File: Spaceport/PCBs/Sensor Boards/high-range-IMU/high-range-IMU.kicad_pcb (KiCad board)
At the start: 2 copper layers, 19.5 x 21.5 mm, 4 parts, among them J1 Conn_01x06, U1 ADXL375BCCZ-RL7

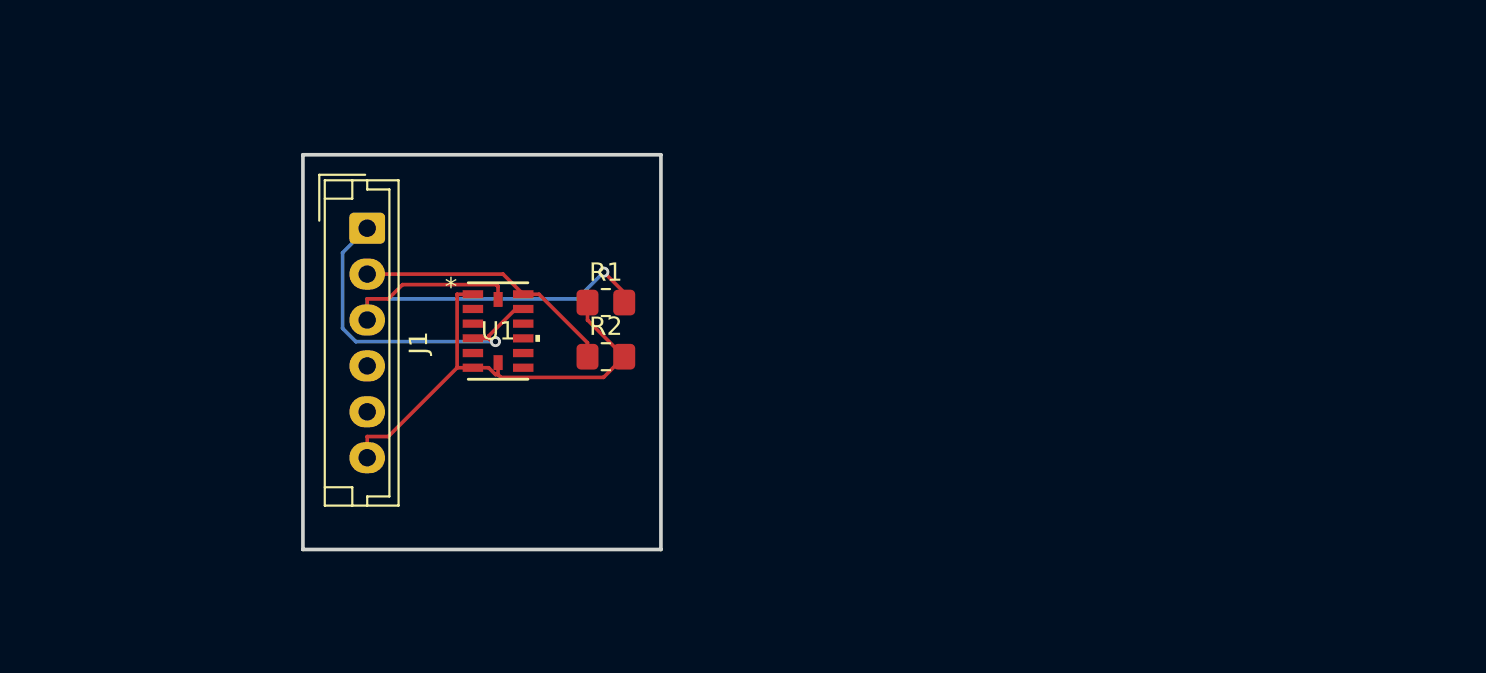
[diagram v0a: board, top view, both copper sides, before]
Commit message: Finished
Don't know if i did the ground plane correct. Don't know if I did the decoupling capacitor circuit correct.
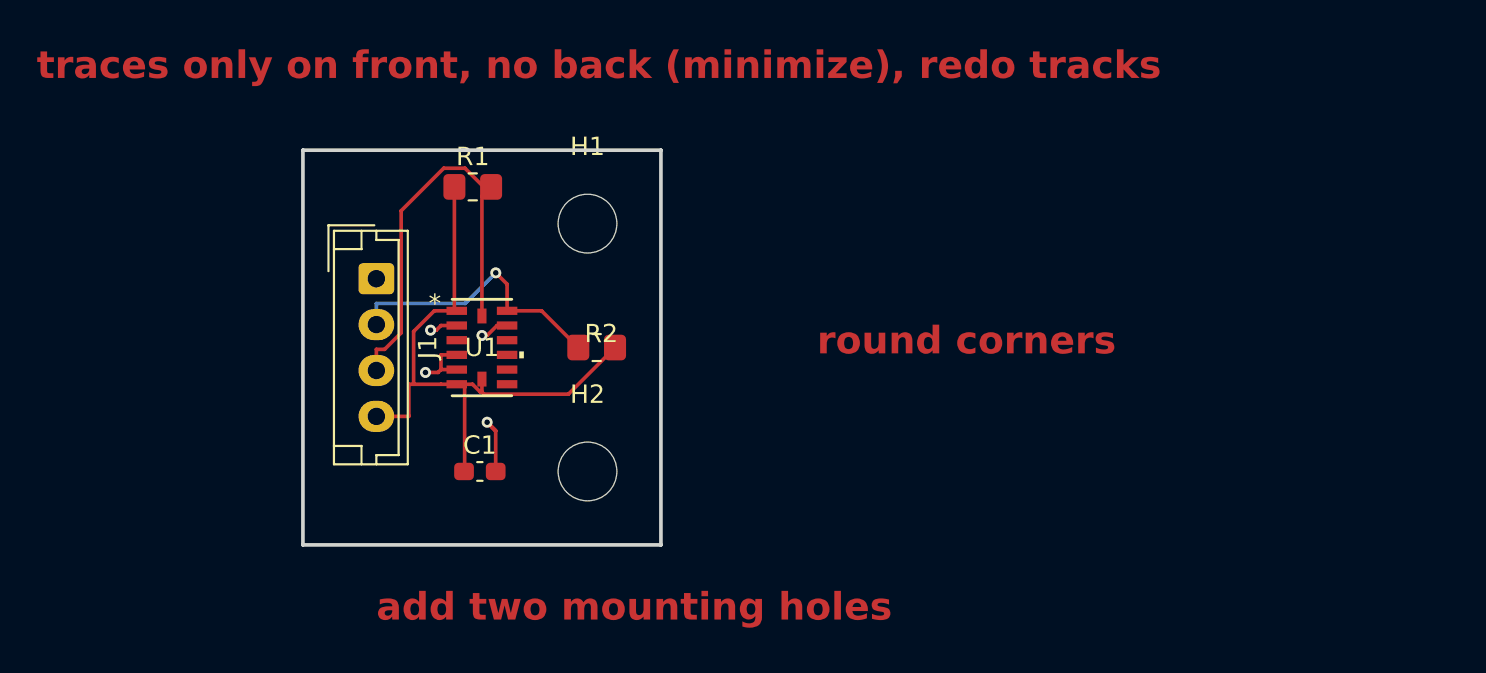
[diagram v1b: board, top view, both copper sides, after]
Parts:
- added C1: C, Capacitor_SMD:C_0603_1608Metric_Pad1.08x0.95mm_HandSolder, F.Cu at (144.6, 95.2)
- added H1: MountingHole, MountingHole:MountingHole_3.2mm_M3, F.Cu at (150.5, 81.8)
- added H2: MountingHole, MountingHole:MountingHole_3.2mm_M3, F.Cu at (150.5, 95.2)
- J1: value Conn_01x06 -> Conn_01x04; footprint Connector_JST:JST_EH_B6B-EH-A_1x06_P2.50mm_Vertical -> Connector_JST:JST_EH_B4B-EH-A_1x04_P2.50mm_Vertical
- moved R1 9.60 mm to (144.2, 79.8)
- moved J1 2.80 mm to (139.0, 84.8)
- moved U1 1.26 mm to (144.8, 88.5)
- moved R2 0.71 mm to (151.0, 88.5)
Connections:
- J1 pad 4: unconnected-(J1-Pin_4-Pad4) -> +3.3V
- U1 pad 2: unconnected-(U1-GND-Pad2) -> GND
- U1 pad 5: unconnected-(U1-GND-Pad5) -> GND
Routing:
- net GND: track 19.4 -> 11.4 mm, vias 1 -> 4
- net +3.3V: track 26.7 -> 33.9 mm
- net Net-(J1-Pin_3): track 26.1 -> 22.9 mm, vias 1 -> 0
- net Net-(J1-Pin_2): track 14.3 -> 15.4 mm, vias 0 -> 1
- added copper zone on B.Cu, net GND
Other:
- board text added: "add two mounting holes"
- board text added: "round corners"
- board text added: "traces only on front, no back (minimize), redo tracks"

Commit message: update PCB layout
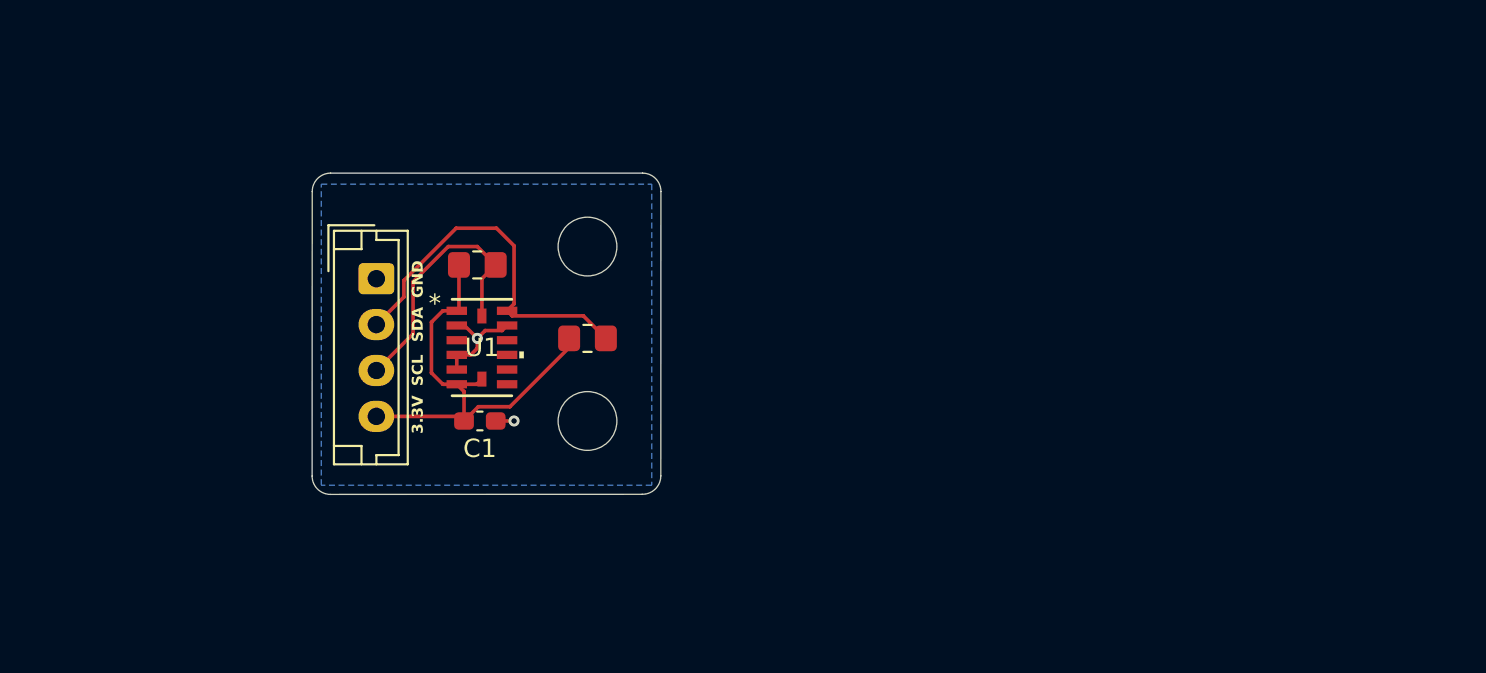
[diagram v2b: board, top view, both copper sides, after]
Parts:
- moved R1 4.26 mm to (144.5, 84.0)
- moved C1 2.75 mm to (144.6, 92.5)
- moved H2 2.75 mm to (150.5, 92.5)
- moved H1 1.25 mm to (150.5, 83.0)
- moved R2 0.71 mm to (150.5, 88.0), turned to 180 degrees
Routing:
- net +3.3V: track 33.9 -> 25.0 mm
- net Net-(J1-Pin_3): track 22.9 -> 14.5 mm
- net Net-(J1-Pin_2): track 15.4 -> 20.3 mm, vias 1 -> 0
- net GND: track 11.4 -> 6.93 mm, vias 4 -> 2
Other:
- board size 19.5 x 21.5 mm -> 19 x 17.5 mm
- board text added: "3.3V"
- board text added: "GND"
- board text added: "SCL"
- board text added: "SDA"
- board text removed: "add two mounting holes"
- board text removed: "round corners"
- board text removed: "traces only on front, no back (minimize), redo tracks"
